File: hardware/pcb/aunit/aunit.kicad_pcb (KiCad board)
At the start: 2 copper layers, 62.2 x 21.6 mm, 48 parts, among them J1 BUS, J2 Input A, J3 Input B, J4 Control, J5 Flags, J6 Power, U1 74HC283, U2 74HC283, U3 74HC86, U4 74HC86, U5 74HC86, U6 74HC08, U7 74HC245, U8 74HC125

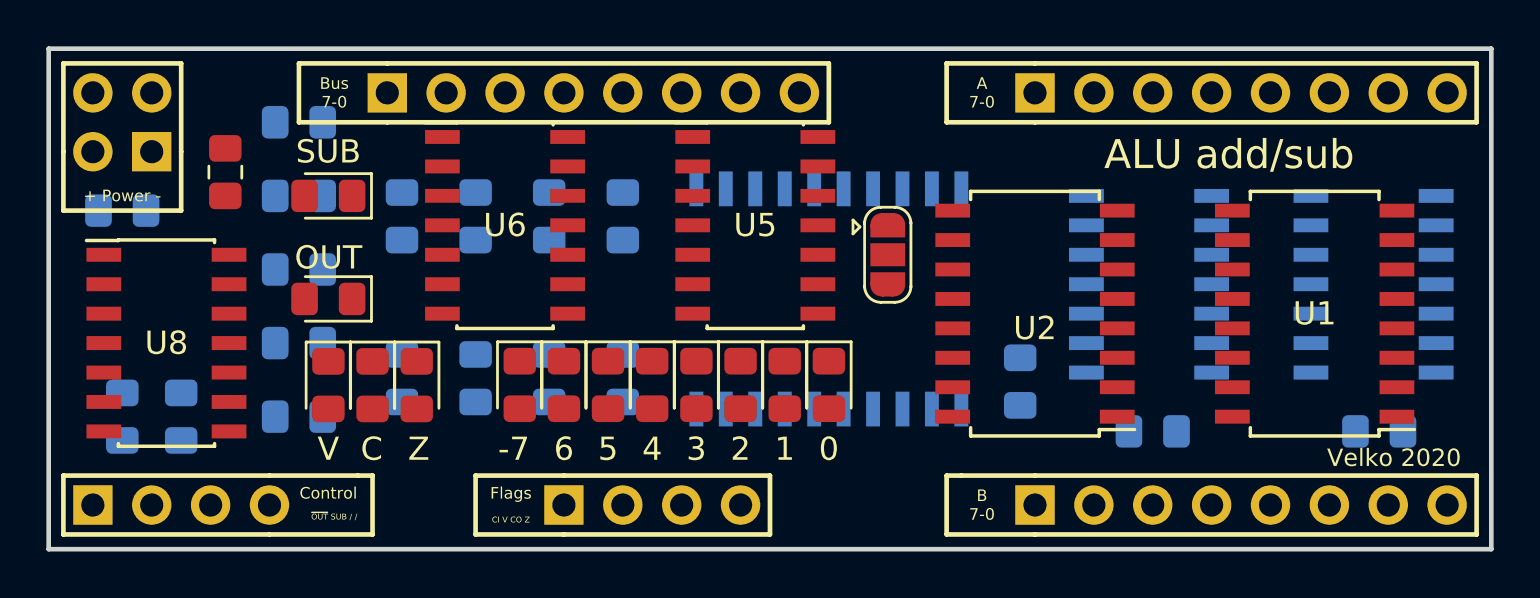
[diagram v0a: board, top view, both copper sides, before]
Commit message: Imported autorouted
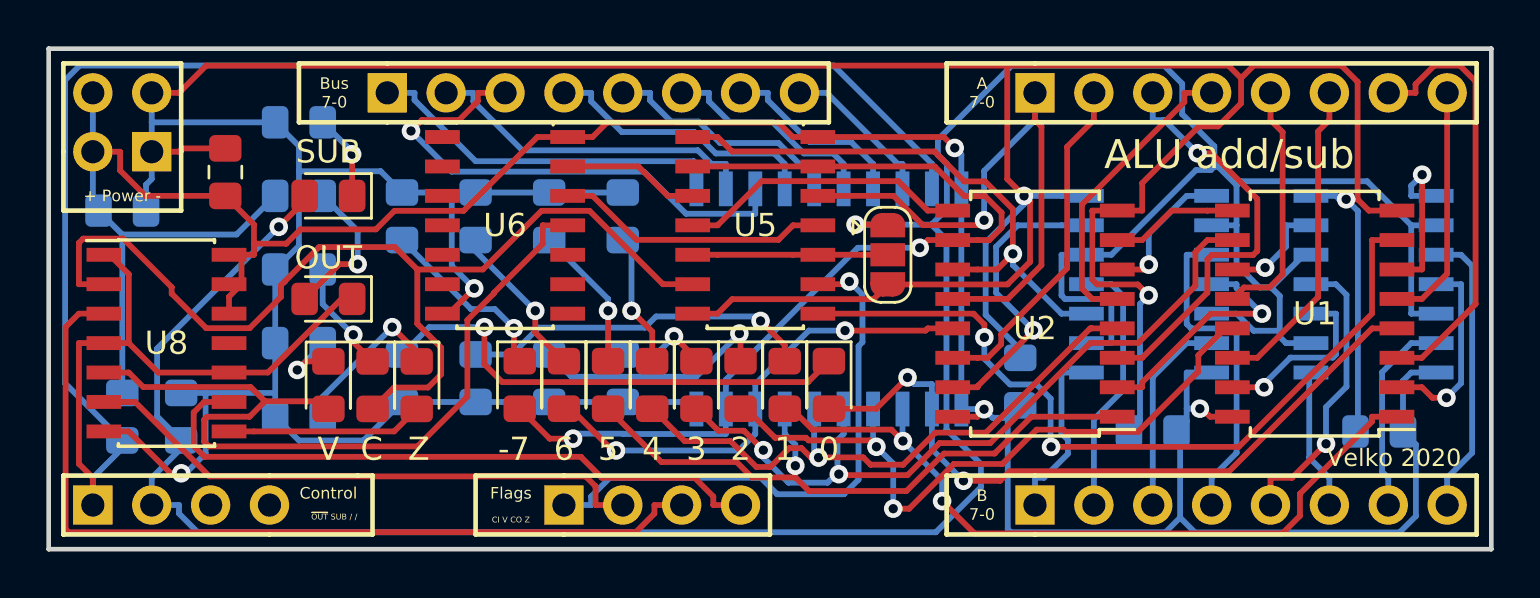
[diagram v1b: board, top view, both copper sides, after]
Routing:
- net GND: track 0.00 -> 209.5 mm, vias 0 -> 5
- net ADD_SUB: track 0.00 -> 137.9 mm, vias 0 -> 2
- net VCC: track 0.00 -> 124.4 mm, vias 0 -> 3
- net ~OUT~: track 0.00 -> 85.6 mm
- net CARRYD: track 0.00 -> 44.2 mm
- net SUM7: track 0.00 -> 41.3 mm, vias 0 -> 2
- net COUT: track 0.00 -> 37.9 mm
- net OVFD: track 0.00 -> 36.4 mm
- net /CII: track 0.00 -> 35.0 mm, vias 0 -> 2
- net SUM1: track 0.00 -> 33.3 mm, vias 0 -> 2
- net SUM3: track 0.00 -> 32.8 mm, vias 0 -> 2
- net SUM0: track 0.00 -> 31.3 mm, vias 0 -> 2
- net SUM2: track 0.00 -> 29.5 mm, vias 0 -> 2
- net ZIN: track 0.00 -> 28.0 mm
- net SUM5: track 0.00 -> 27.9 mm, vias 0 -> 1
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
